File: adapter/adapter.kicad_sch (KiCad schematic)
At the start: 32 parts, among them J1 Serial, J10 Ribbon, J11 Ribbon, J12 Ribbon, J13 serial, J14 serial, J2 Serial, J3 battery charge, J4 RGB, J5 RGB, J6 battery charge, J7 trackball, J8 trackball, J9 Ribbon, SW1 SW_SPST, SW2 SW_SPST, SW3 SW_SPDT, SW4 SW_SPDT, U1 eliteC, U2 eliteC

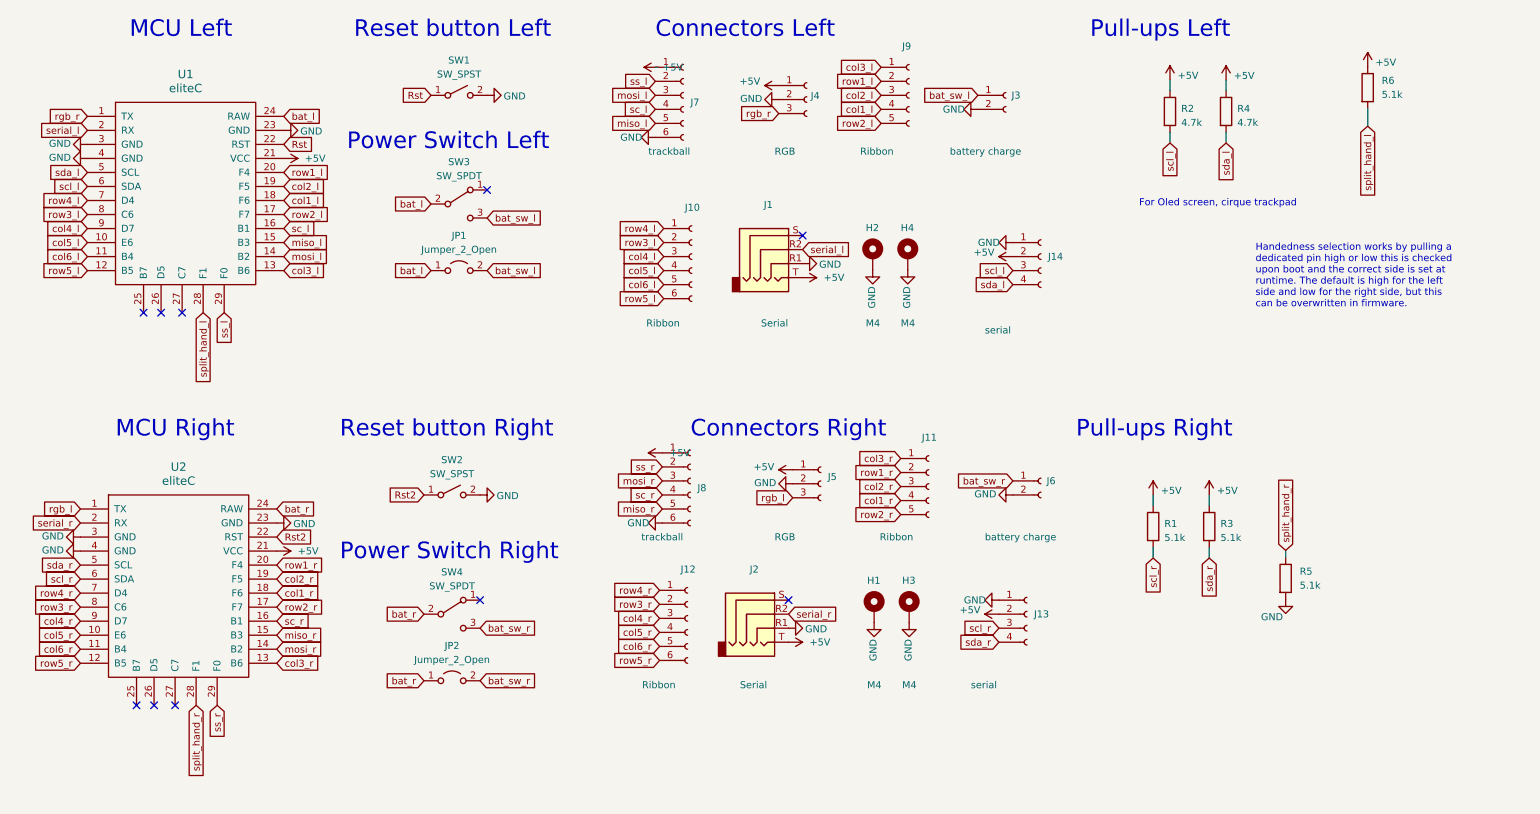
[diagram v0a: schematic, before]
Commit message: routed
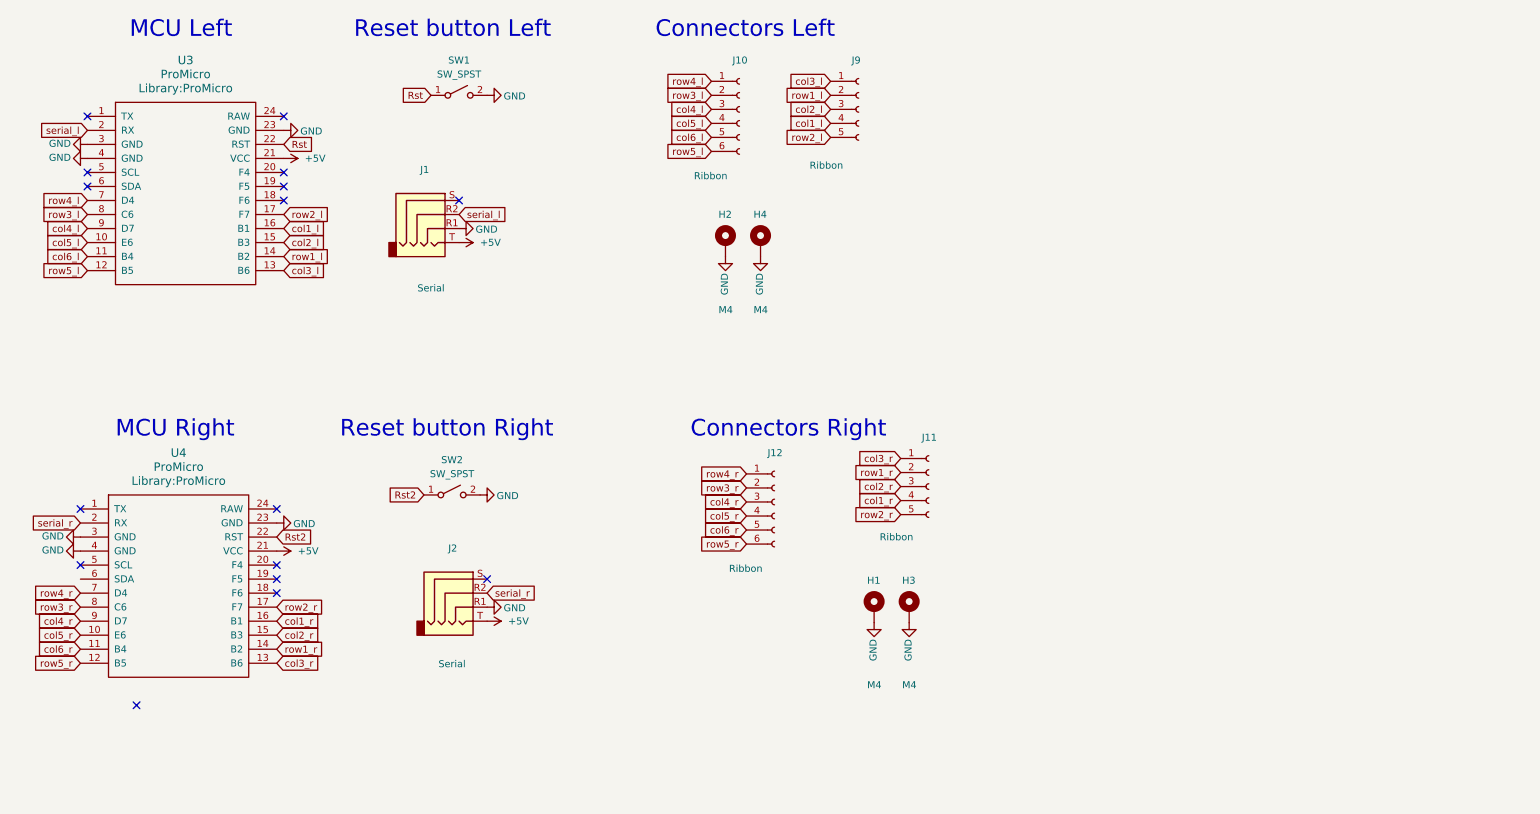
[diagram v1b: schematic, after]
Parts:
- removed J13, J14: serial, Library:PinHeader_1x04_P2.54mm_Vertical, symbol Connector:Conn_01x04_Female
- removed J3, J6: battery charge, Library:PinHeader_1x02_P2.54mm_Vertical, symbol Connector:Conn_01x02_Female
- removed J4, J5: RGB, Library:header1x03, symbol Connector:Conn_01x03_Female
- removed J7, J8: trackball, Library:6_PinHeader, symbol Connector:Conn_01x06_Female
- removed JP1, JP2: Jumper_2_Open, Library:power_switch_jumper, symbol Jumper:Jumper_2_Open
- removed R1, R3, R5, R6: 5.1k, Library:R_1206_handsolder, symbol Device:R
- removed R2, R4: 4.7k, Library:R_1206_handsolder, symbol Device:R
- removed SW3, SW4: SW_SPDT, Library:SW_SPDT+H-MSK12C01_hor(7pin_SMD), symbol Switch:SW_SPDT
- removed U1, U2: eliteC, Library:Elite-C, symbol elite-C:eliteC
- added U3, U4: ProMicro, Library:ProMicro, symbol promicro:ProMicro
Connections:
- net +5V: now also U3.21 (VCC), U4.21 (VCC)
- net GND: now also U3.23 (GND), U3.3 (GND), U3.4 (GND), U4.23 (GND), U4.3 (GND), U4.4 (GND)
- net Rst: now also U3.22 (RST)
- net Rst2: now also U4.22 (RST)
- net col1_l: now also U3.16 (B1)
- net col1_r: now also U4.16 (B1)
- net col2_l: now also U3.15 (B3)
- net col2_r: now also U4.15 (B3)
- net col3_l: now also U3.13 (B6)
- net col3_r: now also U4.13 (B6)
- net col4_l: now also U3.9 (D7)
- net col4_r: now also U4.9 (D7)
- net col5_l: now also U3.10 (E6)
- net col5_r: now also U4.10 (E6)
- net col6_l: now also U3.11 (B4)
- net col6_r: now also U4.11 (B4)
- net row1_l: now also U3.14 (B2)
- net row1_r: now also U4.14 (B2)
- net row2_l: now also U3.17 (F7)
- net row2_r: now also U4.17 (F7)
- net row3_l: now also U3.8 (C6)
- net row3_r: now also U4.8 (C6)
- net row4_l: now also U3.7 (D4)
- net row4_r: now also U4.7 (D4)
- net row5_l: now also U3.12 (B5)
- net row5_r: now also U4.12 (B5)
- net serial_l: now also U3.2 (RX)
- net serial_r: now also U4.2 (RX)
- no-connect marks 10 -> 16
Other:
- note removed: "For Oled screen, cirque trackpad"
- note removed: "Handedness selection works by pulling a dedicated pin high or low this is checked upon boot and the correct side is set at runtime. The default is high for the left side and low for the right side, but this can be overwritten in firmware."
- note removed: "Power Switch Left"
- note removed: "Power Switch Right"
- note removed: "Pull-ups Left"
- note removed: "Pull-ups Right"
- moved on the sheet: H2, H4, J1, J10, J12, J2, J9
